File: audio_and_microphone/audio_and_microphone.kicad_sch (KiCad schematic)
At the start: 15 parts, among them U2 ${SIM.PARAMS}

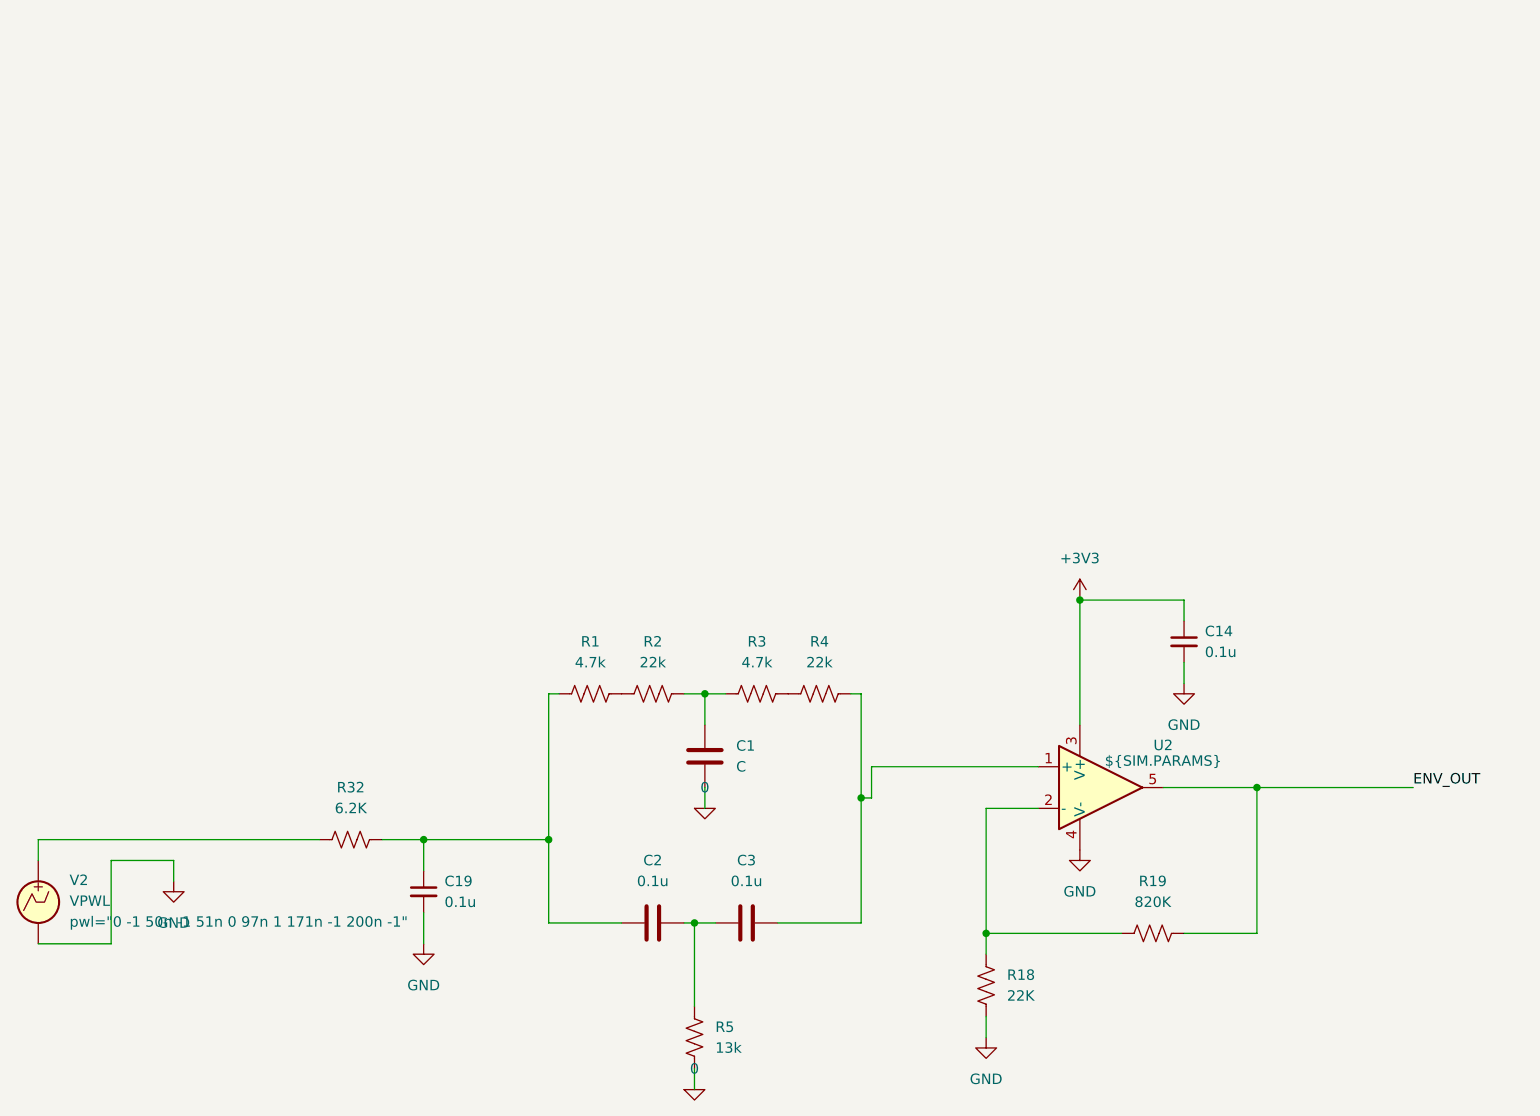
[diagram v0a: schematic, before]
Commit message: created inital pcb layout
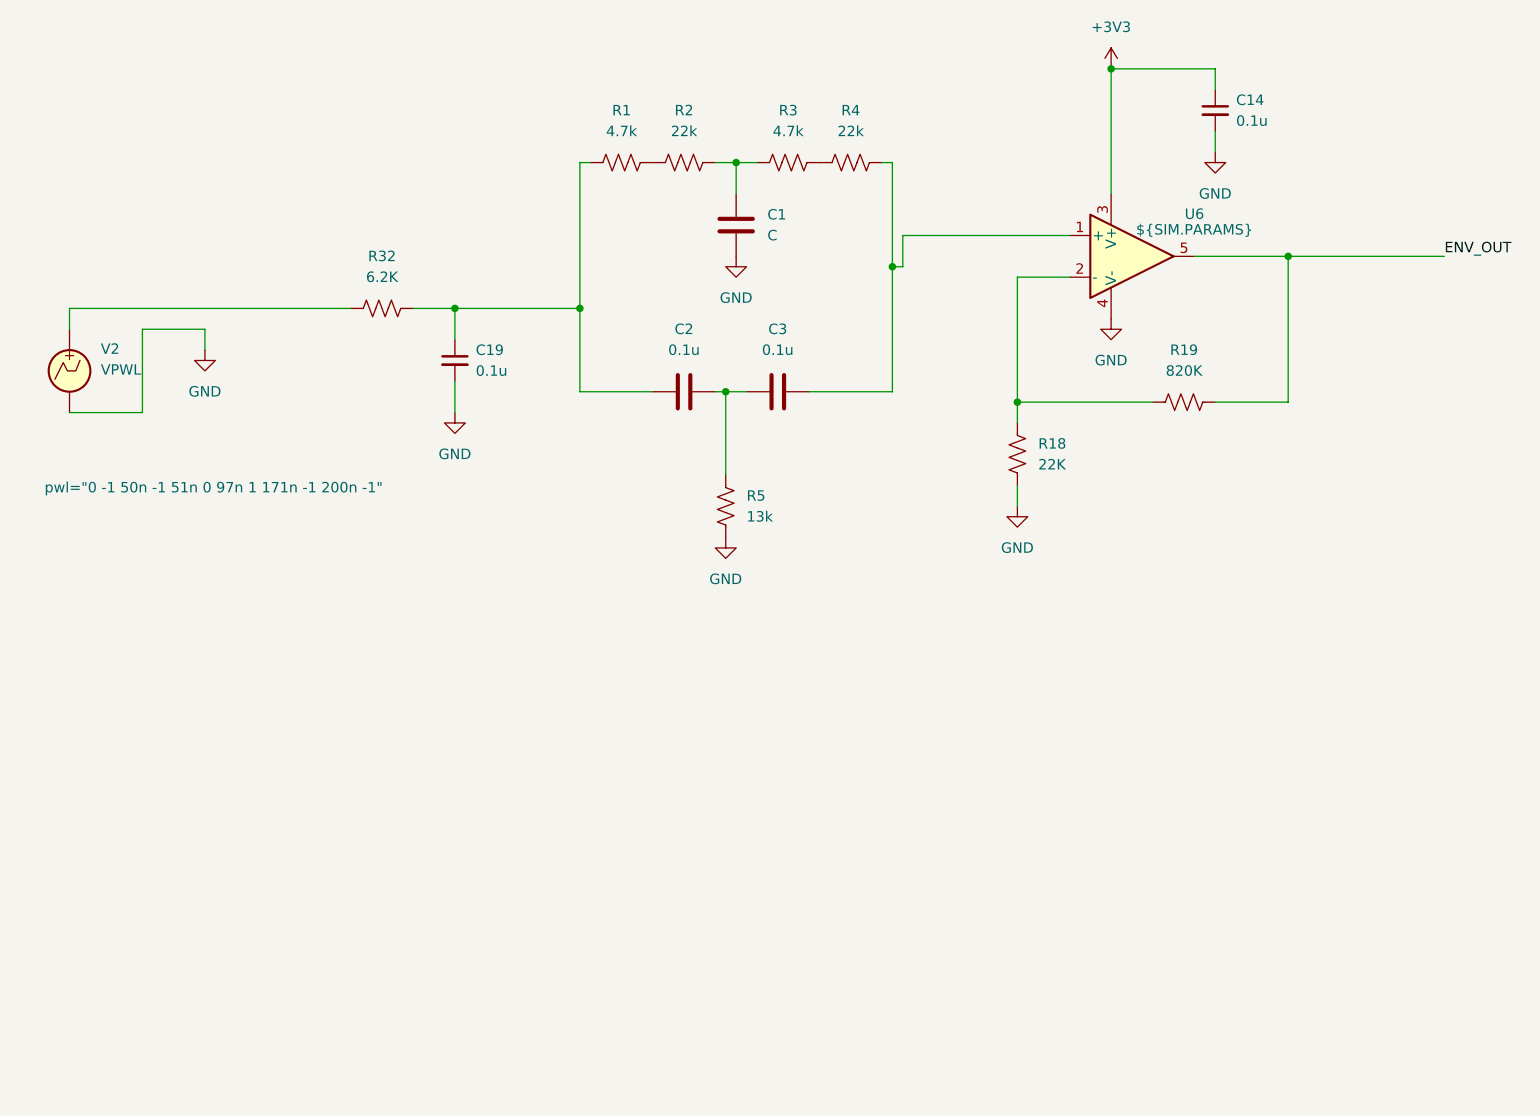
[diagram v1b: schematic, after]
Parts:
- C1, C14, C19, C2, C3: footprint (none) -> Capacitor_SMD:C_0201_0603Metric
- R1, R18, R19, R2, R3, R32, R4, R5: footprint (none) -> Resistor_SMD:R_0201_0603Metric
- U6: renamed from U2; footprint (none) -> Package_TO_SOT_SMD:SOT-23-5
- V2: footprint (none) -> Connector_PinHeader_2.54mm:PinHeader_1x02_P2.54mm_Vertical
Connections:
- net 0 is gone; now on net GND: C1.2, R5.2
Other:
- moved on the sheet: C1, C14, C19, C2, C3, R1, R18, R19, R2, R3, R32, R4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
